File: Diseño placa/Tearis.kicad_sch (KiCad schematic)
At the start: 5 parts, among them J1 Conn_02x20_Odd_Even, U1 RASPBERRY_PI_ZERO_2_W

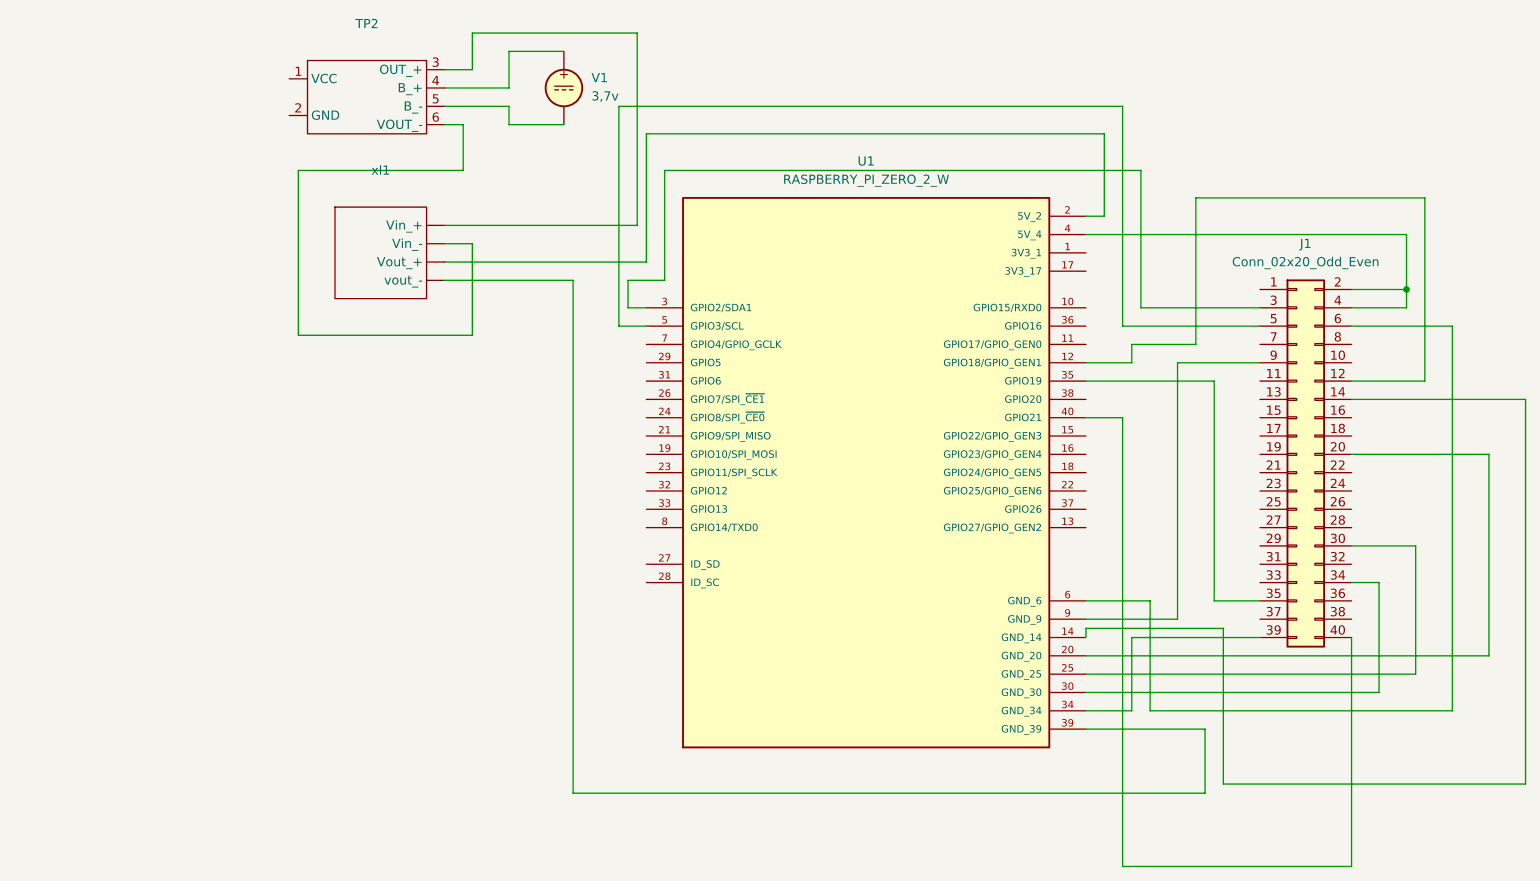
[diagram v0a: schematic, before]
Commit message: actualizacion diseño
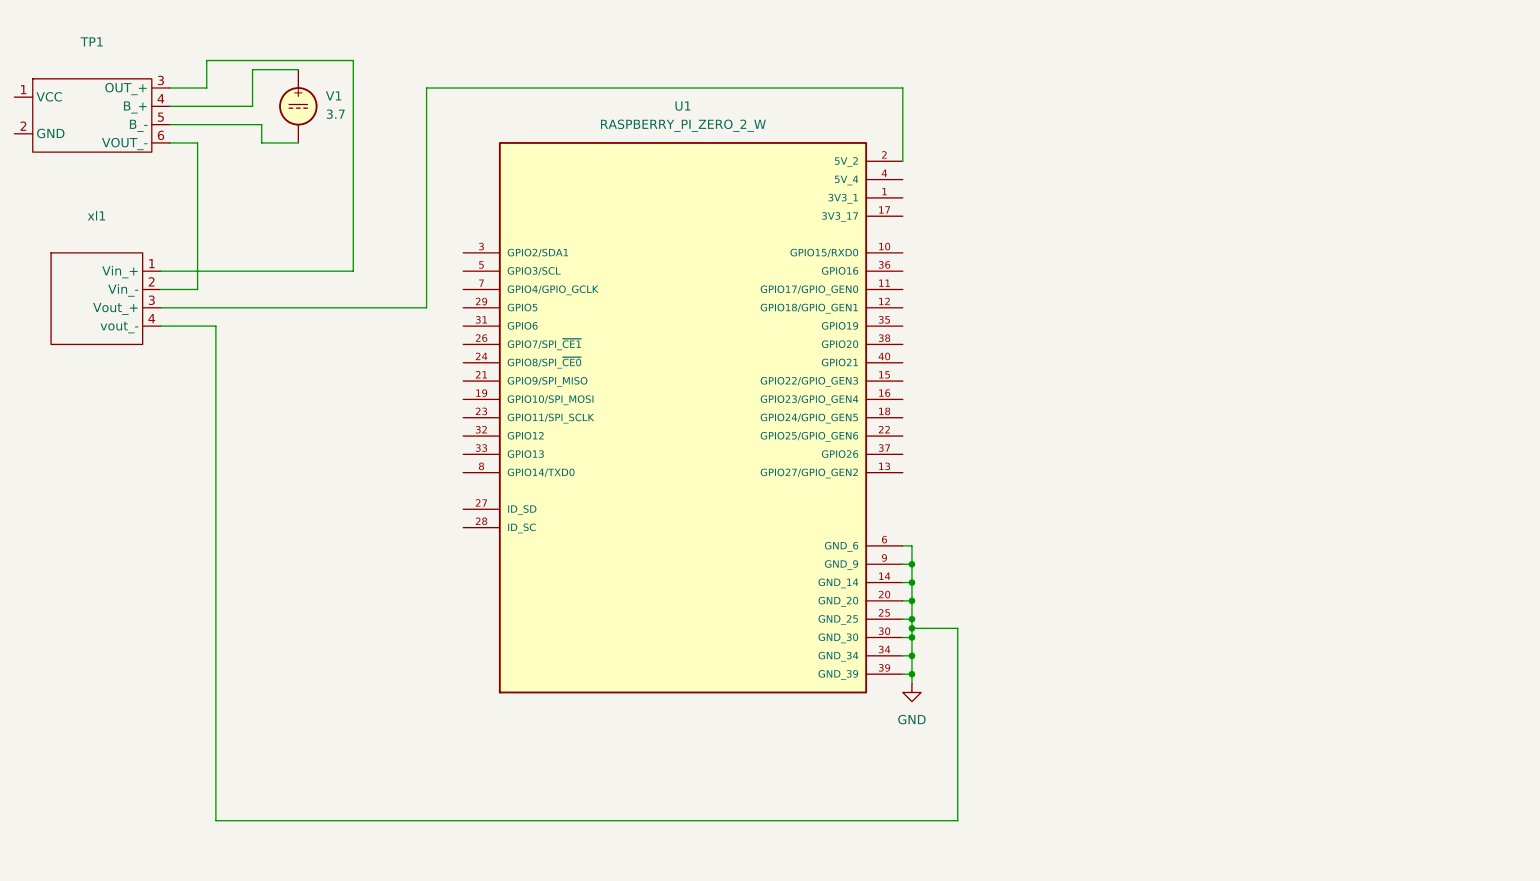
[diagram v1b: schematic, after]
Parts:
- removed J1: Conn_02x20_Odd_Even, symbol Connector_Generic:Conn_02x20_Odd_Even
- removed TP2: ~, symbol Device:TP4056_
- added TP1: ~, Custom_Footprints:TP4056-18650, symbol Device:TP4056_
- U1: footprint RASPBERRY_PI_ZERO_2_W:MODULE_RASPBERRY_PI_ZERO_2_W -> Module:Raspberry_Pi_Zero_Socketed_THT_FaceDown_MountingHoles
- V1: value 3,7v -> 3.7; footprint (none) -> Connector_PinHeader_2.54mm:PinHeader_1x02_P2.54mm_Vertical
- xl1: footprint (none) -> misc_footprints:XL6009_module
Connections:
- net at V1.1: now also TP1.4 (B_+)
- net at V1.2: now also TP1.5 (B_-)
- net GND: now reaches U1.14 (GND_14)
- net GND: now also U1.20 (GND_20), U1.25 (GND_25), U1.30 (GND_30), U1.34 (GND_34), U1.39 (GND_39), U1.6 (GND_6), U1.9 (GND_9), xl1.4 (vout_-)
- net at U1.2 (5V_2): now also xl1.3 (Vout_+); no longer xl1. (vout_-)
- new net: TP1.3 (OUT_+), xl1.1 (Vin_+)
- new net: TP1.6 (VOUT_-), xl1.2 (Vin_-)

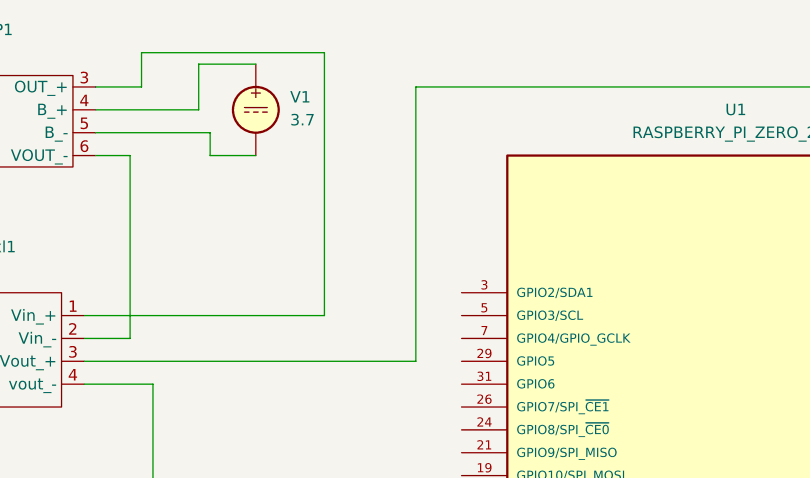
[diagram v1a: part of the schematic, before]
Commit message: actualización placa
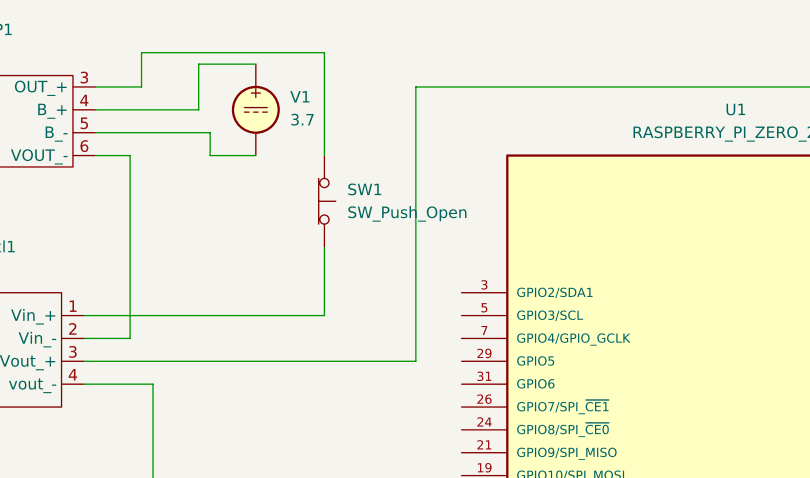
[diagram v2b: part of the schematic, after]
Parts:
- added SW1: SW_Push_Open, TestPoint:TestPoint_2Pads_Pitch5.08mm_Drill1.3mm, symbol Switch:SW_Push_Open
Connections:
- net at TP1.3 (OUT_+): now also SW1.1 (A); no longer xl1.1 (Vin_+)
- new net: SW1.2 (B), xl1.1 (Vin_+)
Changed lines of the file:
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@@
+	(wire
+		(pts
+			(xy 71.12 33.02) (xy 71.12 44.45)
+		)
+		(stroke
+			(width 0)
+			(type default)
+		)
+	)
 	(wire
 		(pts
@@
 	(wire
 		(pts
-			(xy 71.12 33.02) (xy 71.12 62.23)
+			(xy 71.12 54.61) (xy 71.12 62.23)
 		)
 		(stroke
@@
 					(unit 1)
 				)
+			)
+		)
+	)
+	(symbol
+		(lib_id "Switch:SW_Push_Open")
+		(at 71.12 49.53 270)
+		(unit 1)
+		(exclude_from_sim no)
+		(in_bom yes)
+		(on_board yes)
+		(dnp no)
+		(fields_autoplaced yes)
+		(property "Reference" "SW1"
+			(at 73.66 48.2599 90)
+			(effects
+				(font
+					(size 1.27 1.27)
+				)
+				(justify left)
+			)
+		)
+		(property "Value" "SW_Push_Open"
+			(at 73.66 50.7999 90)
+			(effects
+				(font
+					(size 1.27 1.27)
+				)
+				(justify left)
+			)
+		)
+		(property "Footprint" "TestPoint:TestPoint_2Pads_Pitch5.08mm_Drill1.3mm"
+			(at 76.2 49.53 0)
+			(effects
+				(font
+					(size 1.27 1.27)
+				)
+				(hide yes)
+			)
+		)
+		(property "Datasheet" "~"
+			(at 76.2 49.53 0)
+			(effects
+				(font
+					(size 1.27 1.27)
+				)
+				(hide yes)
+			)
+		)
+		(property "Description" "Push button switch, push-to-open, generic, two pins"
+			(at 71.12 49.53 0)
+			(effects
+				(font
+					(size 1.27 1.27)
+				)
+				(hide yes)
+			)
+		)
+		(pin "2"
+		)
+		(pin "1"
+		)
+		(instances
+			(project ""
+				(path "/74b37e89-bb8c-4e65-b16d-a81d9b1b4f58"
+					(reference "SW1")
+					(unit 1)
+				)
